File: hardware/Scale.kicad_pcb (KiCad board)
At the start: 2 copper layers, 45 x 45 mm, 161 parts, among them J1 Load Cell Connector, J2 GPIO, J3 RS232, J4 DebugEdge_02x03, J5 Display Connector, J7 12401610E4#2A, Q1 DMG2307L, Q2 DMG2307L, Q3 BSD235N, SW1 RESET, U1 STM32G070CBTx_u, U10 MCP6001-OT, U2 MCP3562R-E/ST, U3 MCP6N11-010, U4 MCP4542, U7 AP9101CK, U8 MIC5504-3.3YM5, U9 MCP6001-OT, X1 KC2520Z

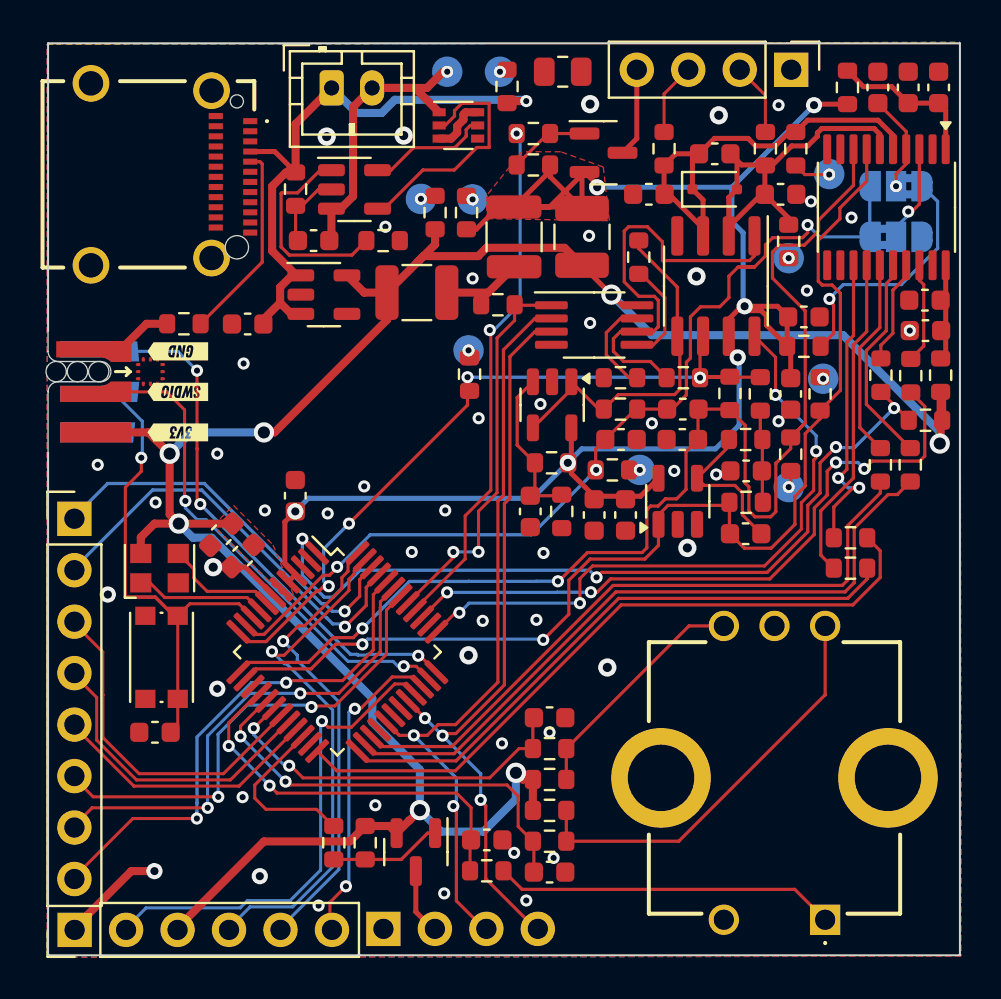
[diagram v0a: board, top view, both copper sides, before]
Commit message: Added net classes
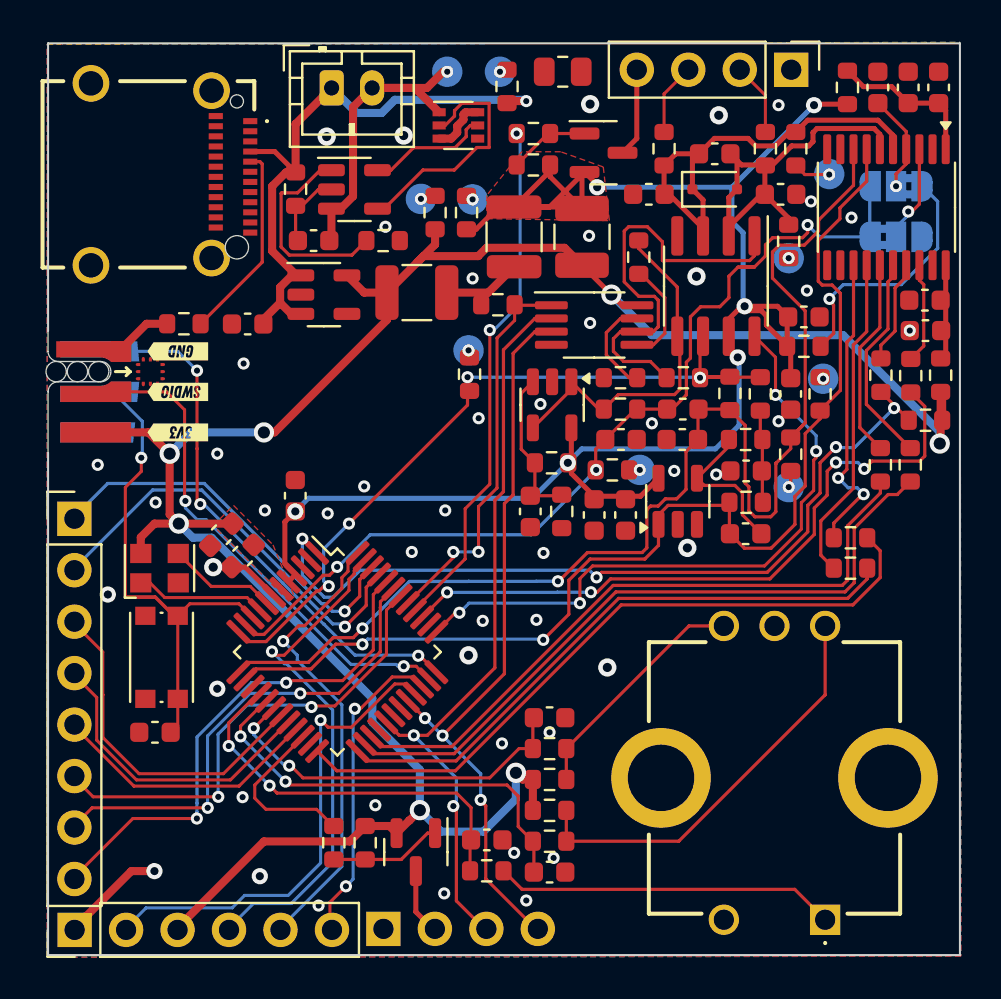
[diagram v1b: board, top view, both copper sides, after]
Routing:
- net /Display/SCL: track 37.5 -> 37.0 mm
